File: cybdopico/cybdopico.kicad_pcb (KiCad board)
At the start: 2 copper layers, 21 x 51 mm, 35 parts, among them P1 USB_C_Plug_USB2.0, SW1 BOOTSEL, SW2 RESET, SW3 HC FLAG, U1 RP2040, U2 USBLC6-2SC6, U3 W25Q16JVUXIQ, U4 MCP1700x-330xxTT, Y1 ABM8-272-T3

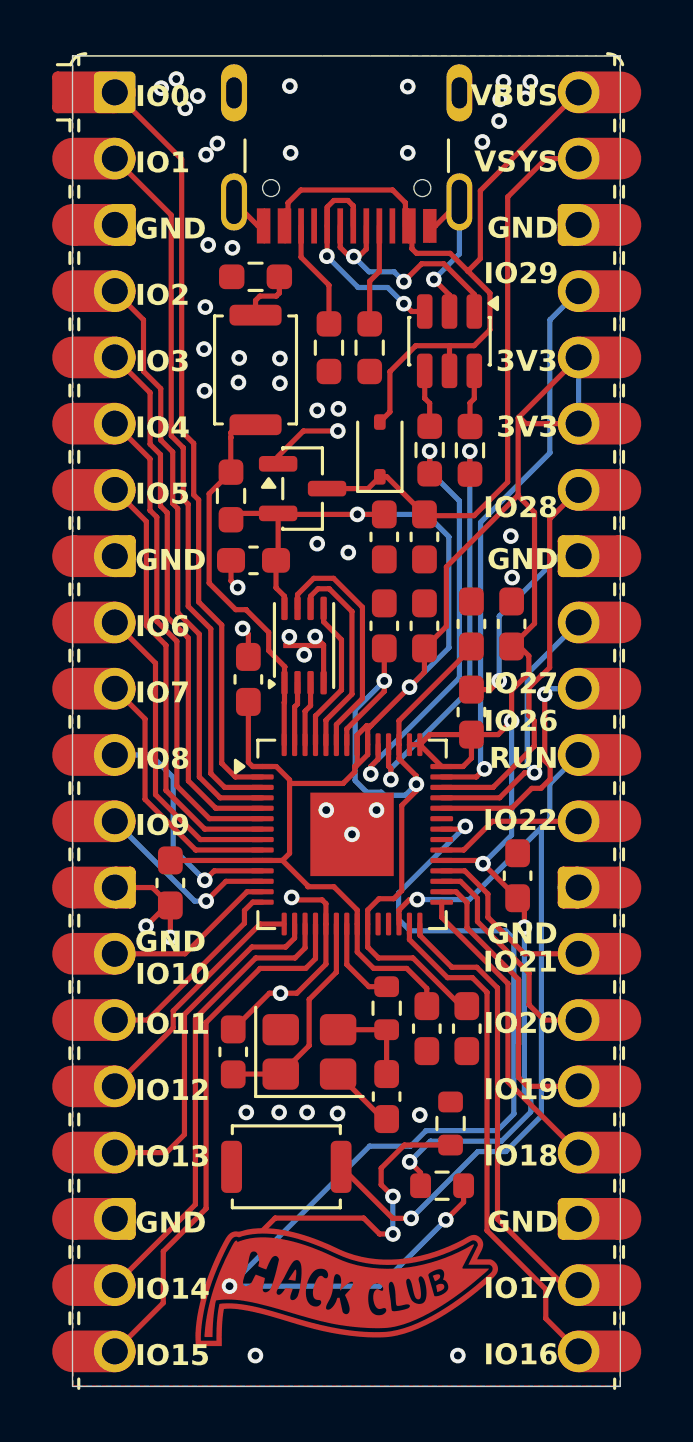
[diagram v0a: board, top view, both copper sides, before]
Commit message: made production files
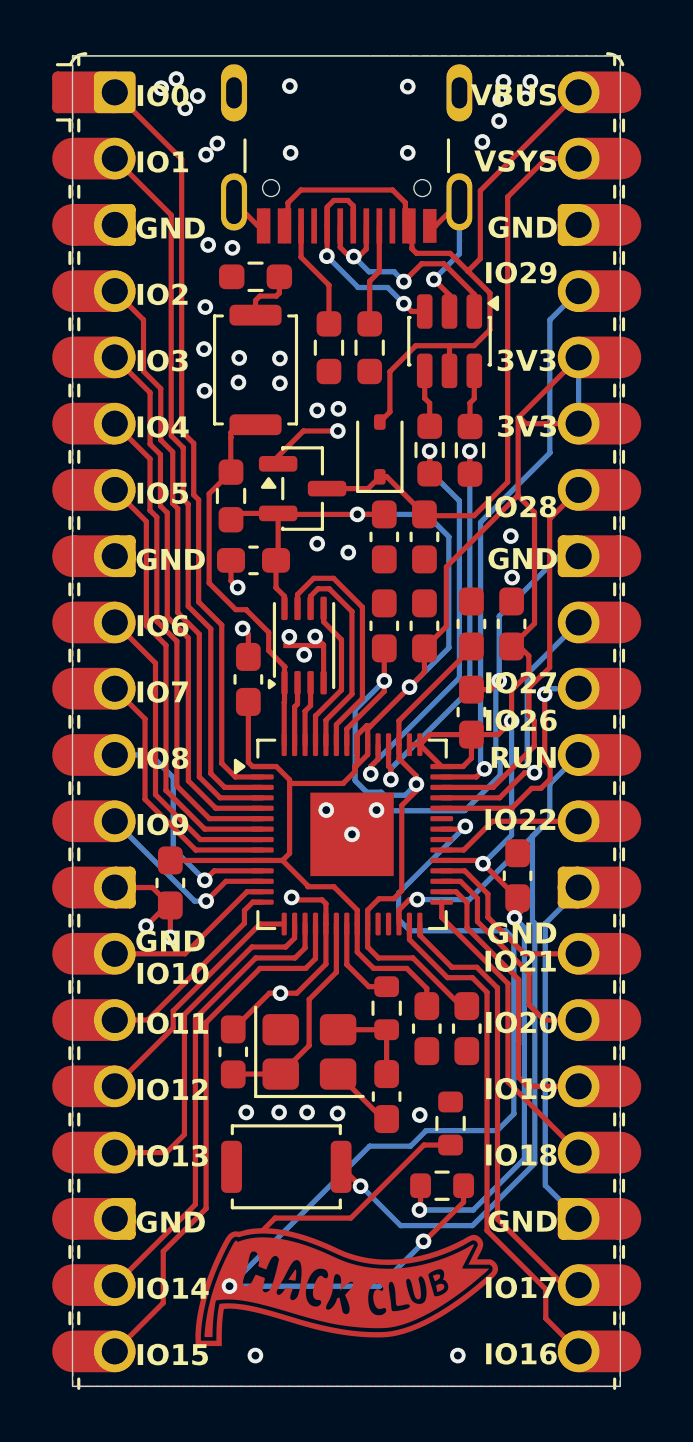
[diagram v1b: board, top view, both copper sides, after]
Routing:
- net GND: track 38.1 -> 62.2 mm
- net Net-(R8-Pad1): track 11.3 -> 8.54 mm, vias 2 -> 0
- net +3V3: track 110.8 -> 112.0 mm
- net RUN: track 31.8 -> 33.1 mm
